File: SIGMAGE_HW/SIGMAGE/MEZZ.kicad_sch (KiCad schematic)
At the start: 4 parts, among them J12 61306421821, J13 61306421121, J14 61306421821, J8 61306421121

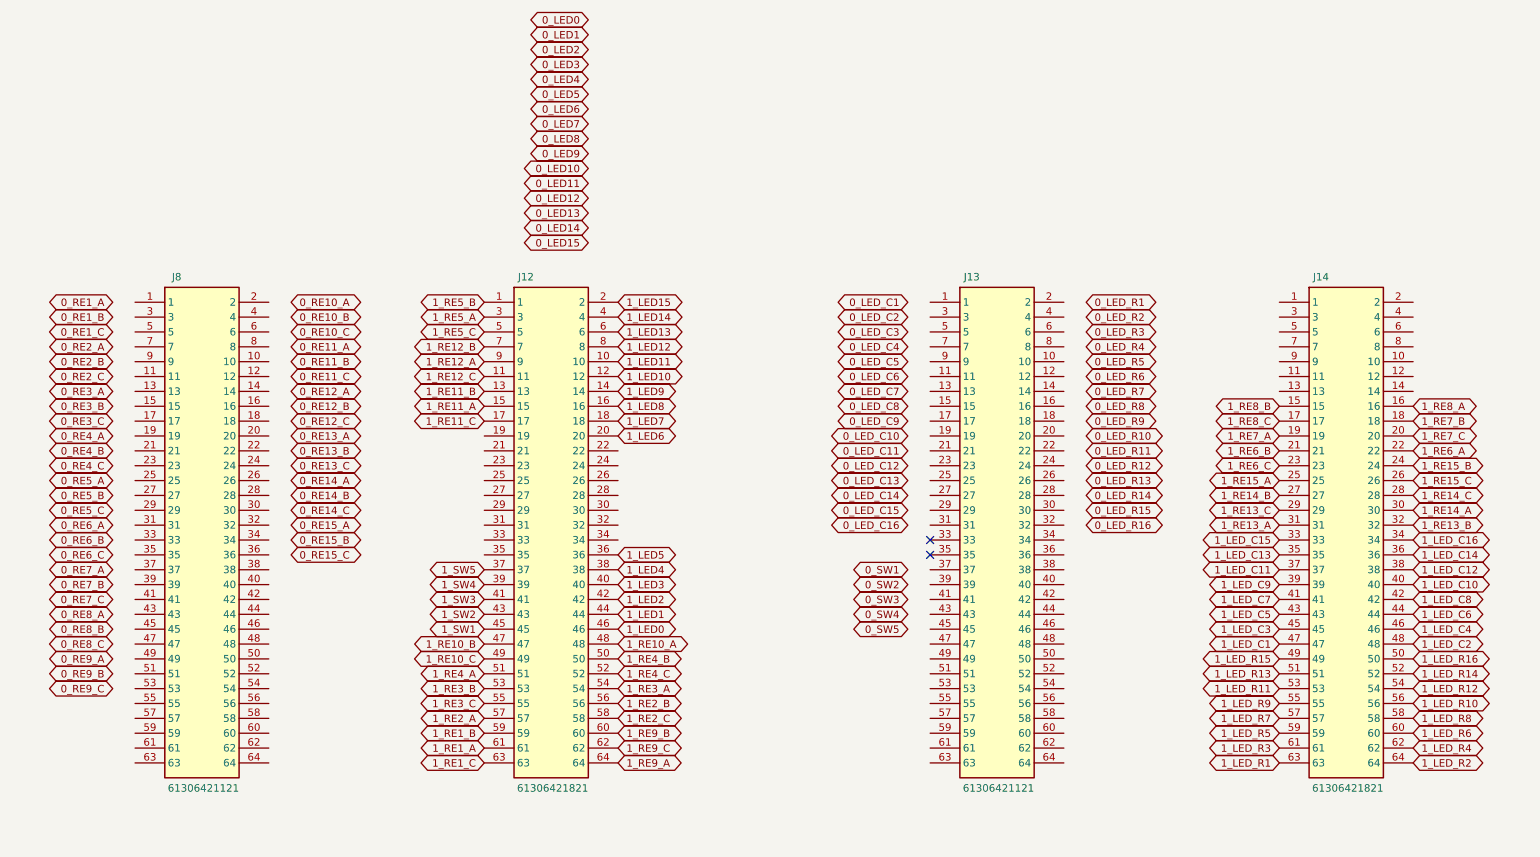
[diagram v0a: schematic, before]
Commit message: almost done with tha top part
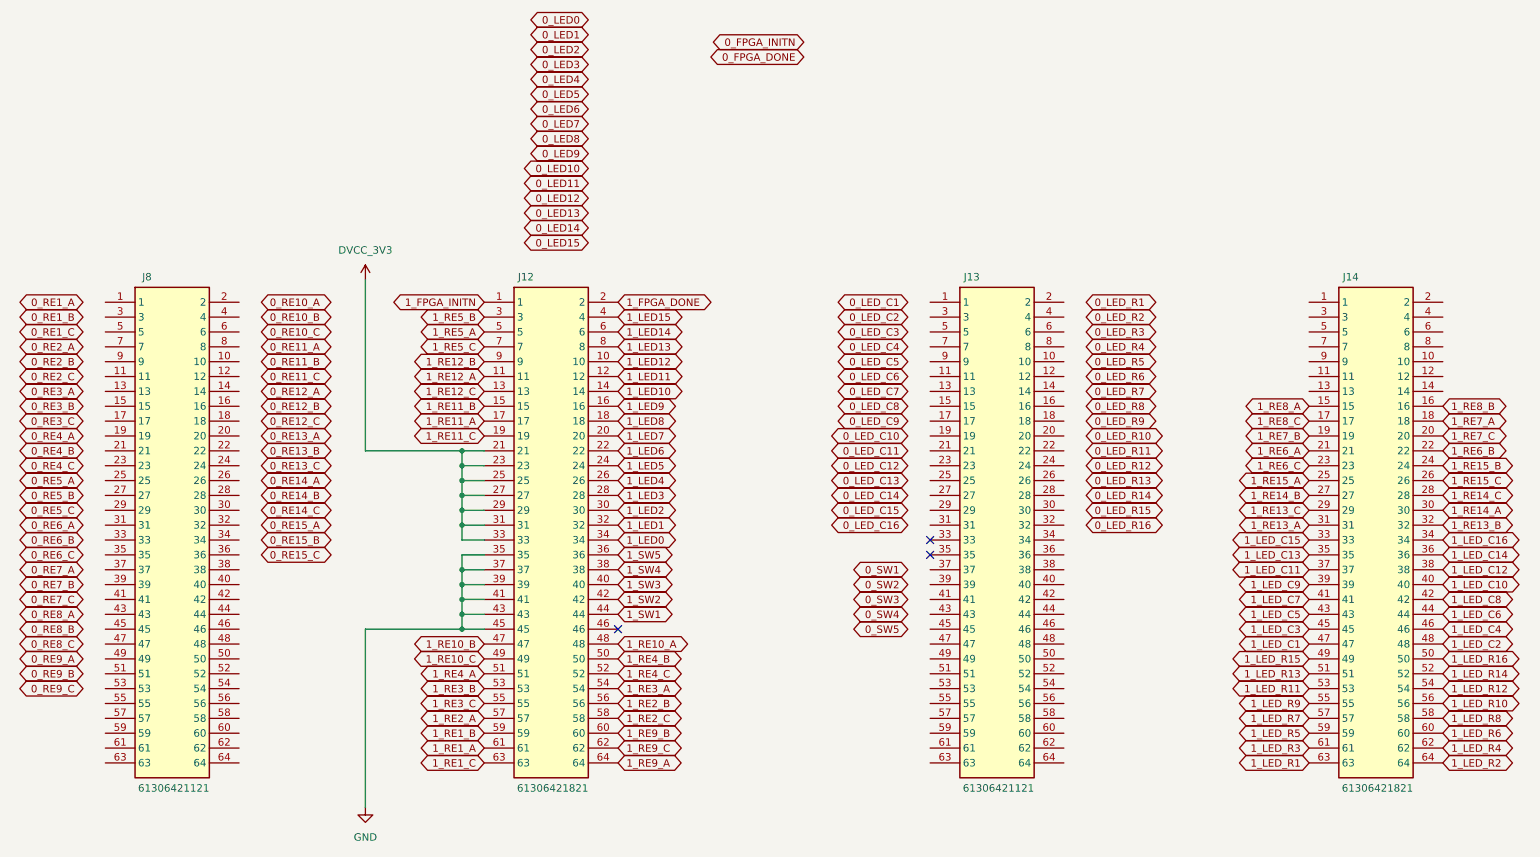
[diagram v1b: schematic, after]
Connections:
- net 1_LED0: now also J12.34; no longer J12.46
- net 1_LED1: now also J12.32; no longer J12.44
- net 1_LED10: now also J12.14; no longer J12.12
- net 1_LED11: now also J12.12; no longer J12.10
- net 1_LED12: now also J12.10; no longer J12.8
- net 1_LED13: now also J12.8; no longer J12.6
- net 1_LED14: now also J12.6; no longer J12.4
- net 1_LED15: now also J12.4; no longer J12.2
- net 1_LED2: now also J12.30; no longer J12.42
- net 1_LED3: now also J12.28; no longer J12.40
- net 1_LED4: now also J12.26; no longer J12.38
- net 1_LED5: now also J12.24; no longer J12.36
- net 1_LED6: now also J12.22; no longer J12.20
- net 1_LED7: now also J12.20; no longer J12.18
- net 1_LED8: now also J12.18; no longer J12.16
- net 1_LED9: now also J12.16; no longer J12.14
- net 1_RE11_A: now also J12.17; no longer J12.15
- net 1_RE11_B: now also J12.15; no longer J12.13
- net 1_RE11_C: now also J12.19; no longer J12.17
- net 1_RE12_A: now also J12.11; no longer J12.9
- net 1_RE12_B: now also J12.9; no longer J12.7
- net 1_RE12_C: now also J12.13; no longer J12.11
- net 1_RE5_A: now also J12.5; no longer J12.3
- net 1_RE5_B: now also J12.3; no longer J12.1
- net 1_RE5_C: now also J12.7; no longer J12.5
- net 1_RE6_A: now also J14.21; no longer J14.22
- net 1_RE6_B: now also J14.22; no longer J14.21
- net 1_RE7_A: now also J14.18; no longer J14.19
- net 1_RE7_B: now also J14.19; no longer J14.18
- net 1_RE8_A: now also J14.15; no longer J14.16
- net 1_RE8_B: now also J14.16; no longer J14.15
- net 1_SW1: now also J12.44; no longer J12.45
- net 1_SW2: now also J12.42; no longer J12.43
- net 1_SW3: now also J12.40; no longer J12.41
- net 1_SW4: now also J12.38; no longer J12.39
- net 1_SW5: now also J12.36; no longer J12.37
- net DVCC_3V3: now reaches J12.21
- net DVCC_3V3: now also J12.23, J12.25, J12.27, J12.29, J12.31, J12.33
- net GND: now reaches J12.35
- net GND: now also J12.37, J12.39, J12.41, J12.43, J12.45
- new net 1_FPGA_DONE: J12.2
- new net 1_FPGA_INITN: J12.1
- no-connect marks 2 -> 3
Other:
- moved on the sheet: J14, J8
